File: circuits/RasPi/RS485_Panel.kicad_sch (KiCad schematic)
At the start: 43 parts, among them J8 Conn_01x07_MountingPin, Q18 S8550, Q19 S8550, Q20 S8550, Q3 S8550, Q4 S8550, Q5 S8550, U10 MAX3485, U11 MAX3485, U12 MAX3485, U13 MAX3485, U8 MAX3485, U9 MAX3485

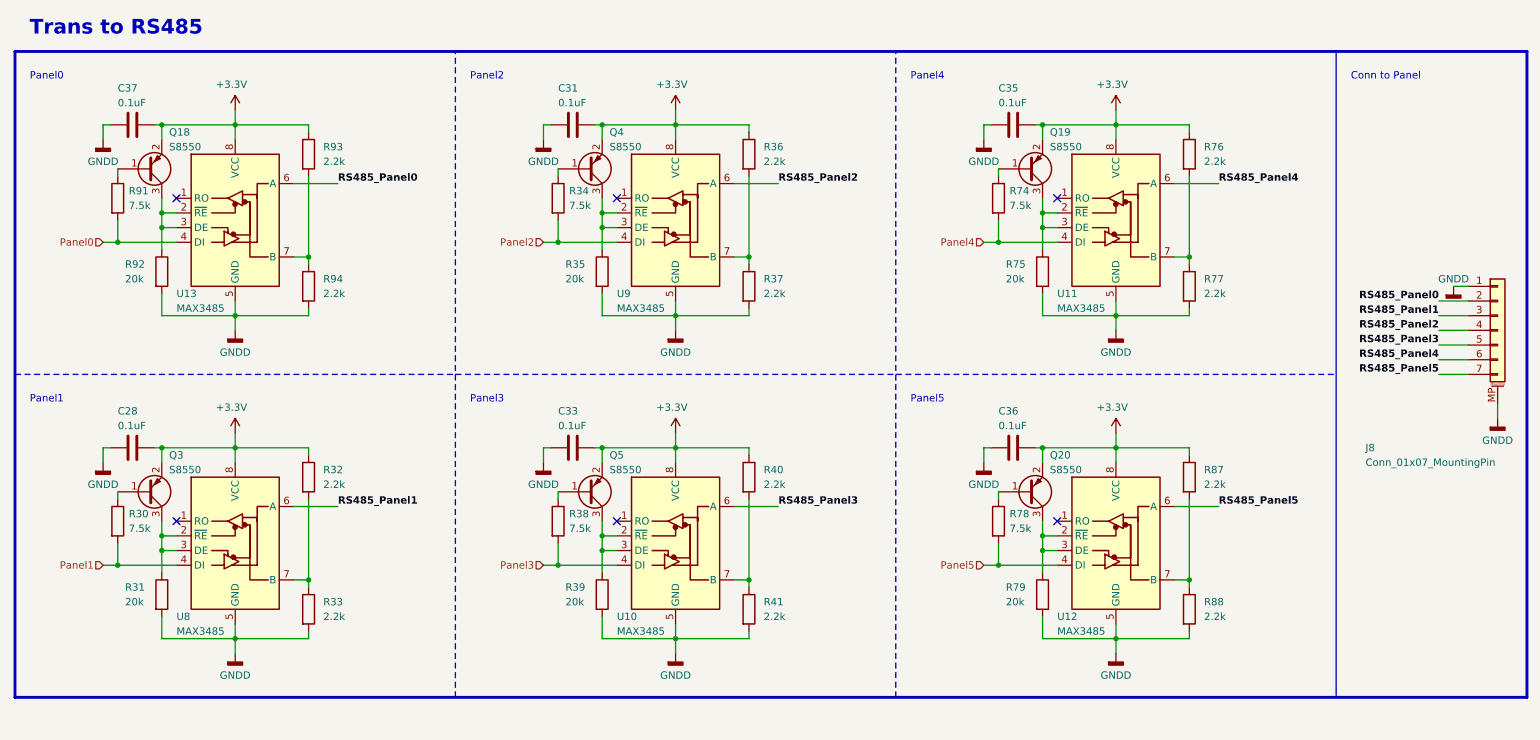
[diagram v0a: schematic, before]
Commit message: PDFプロット
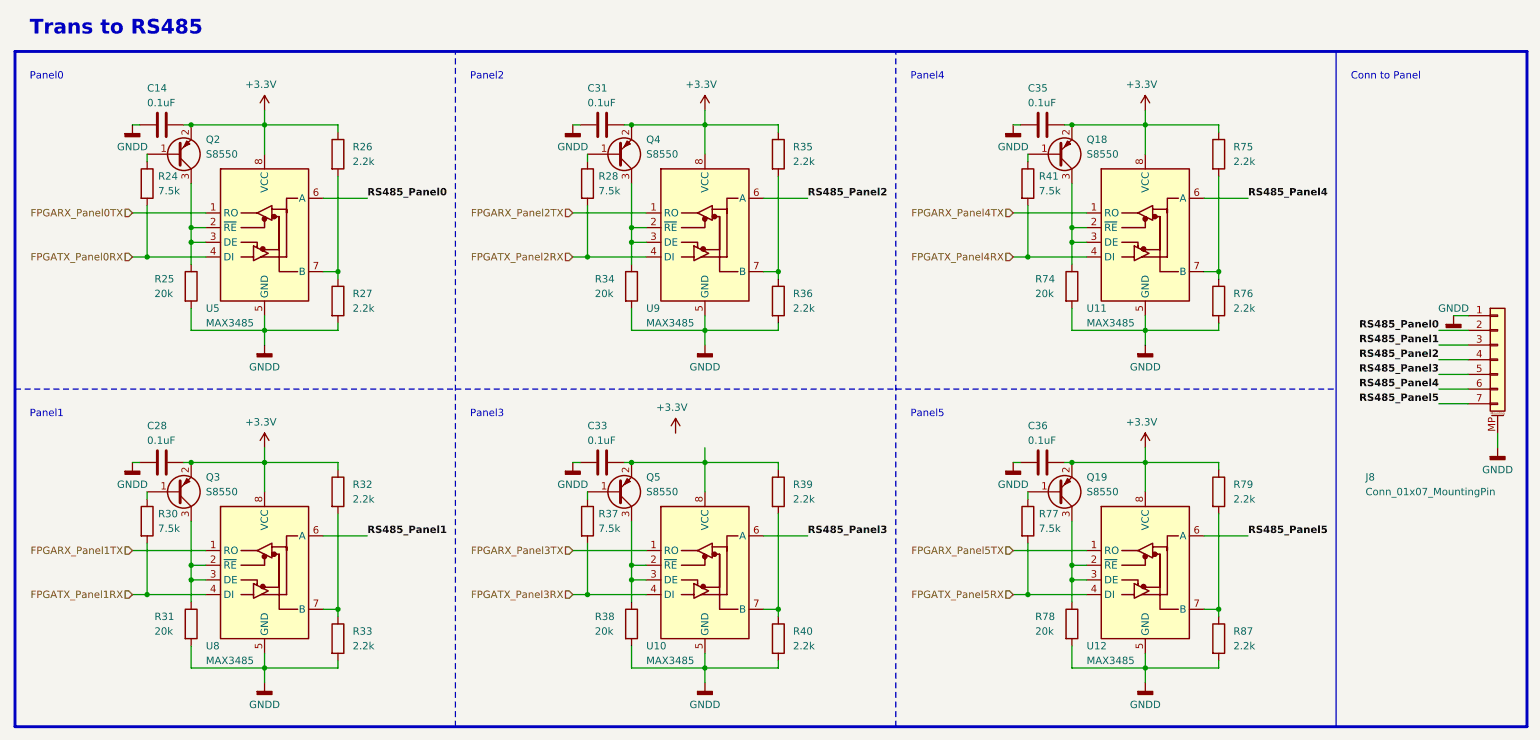
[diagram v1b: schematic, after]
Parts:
- removed C37: 0.1uF, Capacitor_SMD:C_0402_1005Metric, symbol Device:C
- removed Q20: S8550, Package_TO_SOT_SMD:SOT-23, symbol Device:Q_PNP_BEC
- removed R88, R93, R94: 2.2k, Resistor_SMD:R_0402_1005Metric, symbol Device:R
- removed R91: 7.5k, Resistor_SMD:R_0603_1608Metric, symbol Device:R
- removed R92: 20k, Resistor_SMD:R_0402_1005Metric, symbol Device:R
- removed U13: MAX3485, Package_SO:SOP-8_3.9x4.9mm_P1.27mm, symbol Interface_UART:MAX3485
- added C14: 0.1uF, Capacitor_SMD:C_0402_1005Metric, symbol Device:C
- added Q2: S8550, Package_TO_SOT_SMD:SOT-23, symbol Device:Q_PNP_BEC
- added R24, R28: 7.5k, Resistor_SMD:R_0603_1608Metric, symbol Device:R
- added R25: 20k, Resistor_SMD:R_0402_1005Metric, symbol Device:R
- added R26, R27: 2.2k, Resistor_SMD:R_0402_1005Metric, symbol Device:R
- added U5: MAX3485, Package_SO:SOP-8_3.9x4.9mm_P1.27mm, symbol Interface_UART:MAX3485
- J8: footprint (none) -> Connector_Molex:Molex_PicoBlade_53261-0771_1x07-1MP_P1.25mm_Horizontal
- R34, R38, R74, R78: value 7.5k -> 20k; footprint Resistor_SMD:R_0603_1608Metric -> Resistor_SMD:R_0402_1005Metric
- R35, R39, R75, R79: value 20k -> 2.2k
- R37, R41, R77: value 2.2k -> 7.5k; footprint Resistor_SMD:R_0402_1005Metric -> Resistor_SMD:R_0603_1608Metric
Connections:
- net +3.3V: now also R35.1, R75.1, R79.1, C14.1, Q2.2 (E), R26.1, U5.8 (VCC); no longer C33.1, Q5.2 (E), R36.1, R40.1, R76.1, R87.1, U10.8 (VCC)
- net GNDD: now also R34.2, R36.2, R38.2, R40.2, R74.2, R76.2, R78.2, R87.2, C14.2, R25.2, R27.2, U5.5 (GND); no longer R35.2, R37.2, R39.2, R41.2, R75.2, R77.2, R79.2
- net RS485_Panel0: now also U5.6 (A)
- net at R34.1: now also Q4.3 (C), U9.2 (~{RE}), U9.3 (DE); no longer Q4.1 (B)
- net FPGARX_Panel3TX: now reaches U10.1 (RO)
- net at Q5.3 (C), U10.2 (~{RE}), U10.3 (DE): now also R38.1; no longer R39.1
- net FPGARX_Panel2TX: now reaches U9.1 (RO)
- net at Q18.3 (C): now also R74.1, U11.2 (~{RE}), U11.3 (DE)
- net at U12.7 (B): now also R79.2, R87.1; no longer R87.2
- net at Q18.1 (B): now also R41.1
- net at R78.1: now also Q19.3 (C), U12.2 (~{RE}), U12.3 (DE)
- net FPGARX_Panel5TX: now reaches U12.1 (RO)
- net at Q5.1 (B): now also R37.1; no longer R38.1
- net FPGARX_Panel4TX: now reaches U11.1 (RO)
- net at Q19.1 (B): now also R77.1; no longer R74.1
- net FPGARX_Panel1TX: now reaches U8.1 (RO)
- net Panel1 renamed FPGATX_Panel1RX
- net Panel2 renamed FPGATX_Panel2RX
- net FPGATX_Panel2RX: now also R28.2; no longer R34.2
- net Panel3 renamed FPGATX_Panel3RX
- net FPGATX_Panel3RX: now also R37.2; no longer R38.2
- net Panel4 renamed FPGATX_Panel4RX
- net FPGATX_Panel4RX: now also R41.2; no longer R74.2
- net Panel5 renamed FPGATX_Panel5RX
- net FPGATX_Panel5RX: now also R77.2; no longer R78.2
- new net: R35.2, R36.1, U9.7 (B)
- new net: Q2.1 (B), R24.1
- new net: R39.2, R40.1, U10.7 (B)
- new net: R75.2, R76.1, U11.7 (B)
- new net: C33.1, Q5.2 (E), R39.1, U10.8 (VCC)
- new net: R26.2, R27.1, U5.7 (B)
- new net: Q4.1 (B), R28.1
- new net: Q2.3 (C), R25.1, U5.2 (~{RE}), U5.3 (DE)
- new net FPGARX_Panel0TX: U5.1 (RO)
- new net FPGATX_Panel0RX: R24.2, U5.4 (DI)
- no-connect marks 6 -> 0
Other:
- moved on the sheet: C28, J8, Q3, R30, R31, R32, R33, U8
